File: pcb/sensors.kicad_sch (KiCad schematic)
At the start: 27 parts, among them J2 Conn_01x04, J3 Conn_01x04, J4 6P4C, J5 Conn_02x05_Odd_Even, U3 BME280, U4 SGP41, U6 SN65HVD485EDR, U7 2N7001TDPWR, U8 2N7001TDPWR, U9 2N7001TDPWR

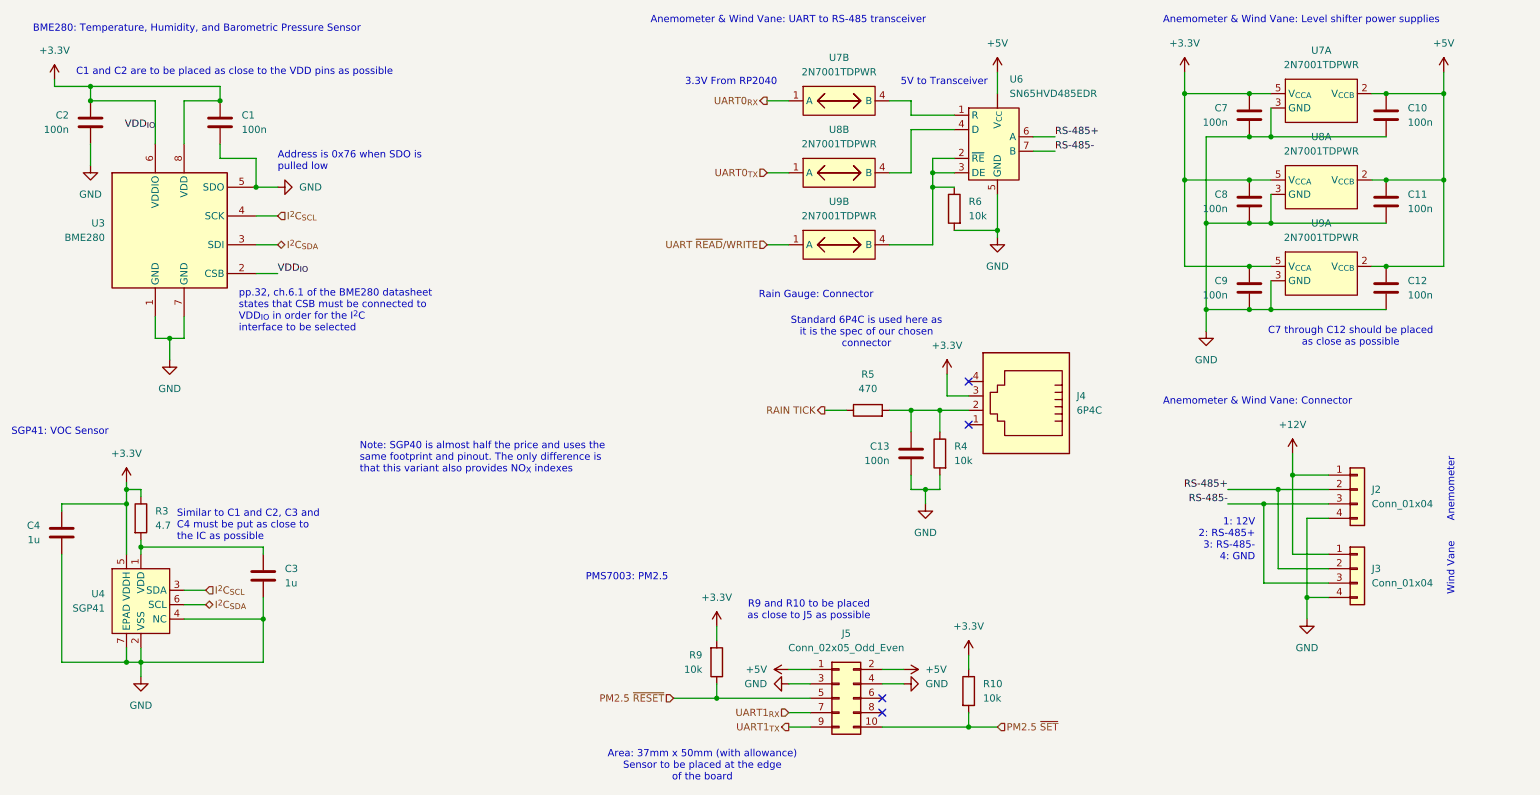
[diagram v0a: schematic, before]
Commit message: feat: finalized usb receptacle
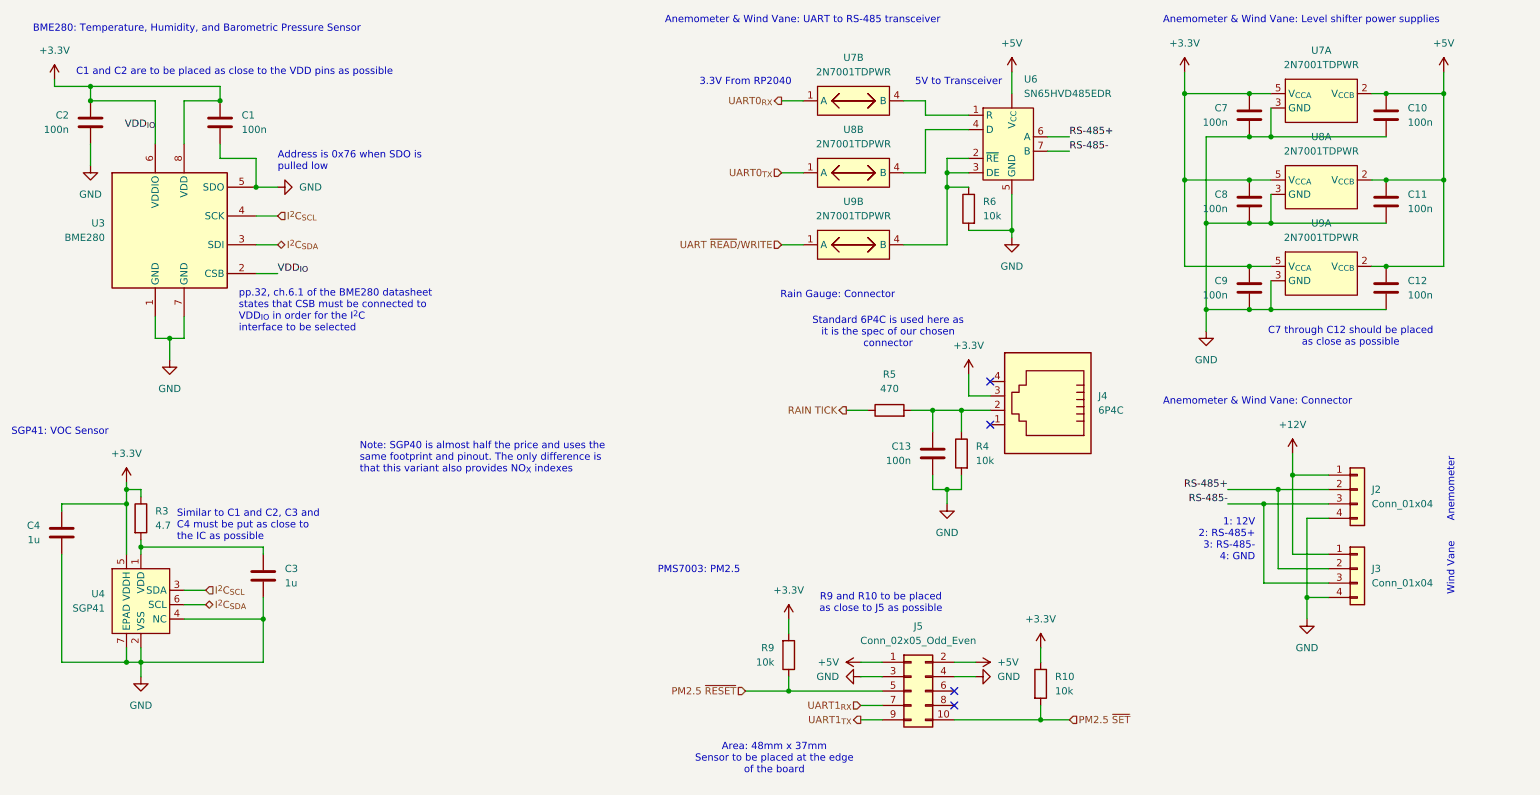
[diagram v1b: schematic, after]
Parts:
- J2, J3: footprint (none) -> Connector_PinHeader_2.54mm:PinHeader_1x04_P2.54mm_Vertical
- J5: footprint (none) -> Connector_PinHeader_1.27mm:PinHeader_2x05_P1.27mm_Vertical
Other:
- note added: "Area: 48mm x 37mm Sensor to be placed at the edge of the board"
- note removed: "Area: 37mm x 50mm (with allowance) Sensor to be placed at the edge of the board"
- moved on the sheet: C13, J4, J5, R10, R4, R5, R6, R9, U6, U7B, U8B, U9B
